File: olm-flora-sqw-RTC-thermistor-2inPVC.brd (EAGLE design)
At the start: 37.3 x 50.8 mm, 33 parts, among them IC1 ATMEGA32U4-AU, IC2 DS3231SN, IC3 MCP73831, IC4 MCP1700-33, J1 AYZ0202, X1 USBSMD, X3 8MHz

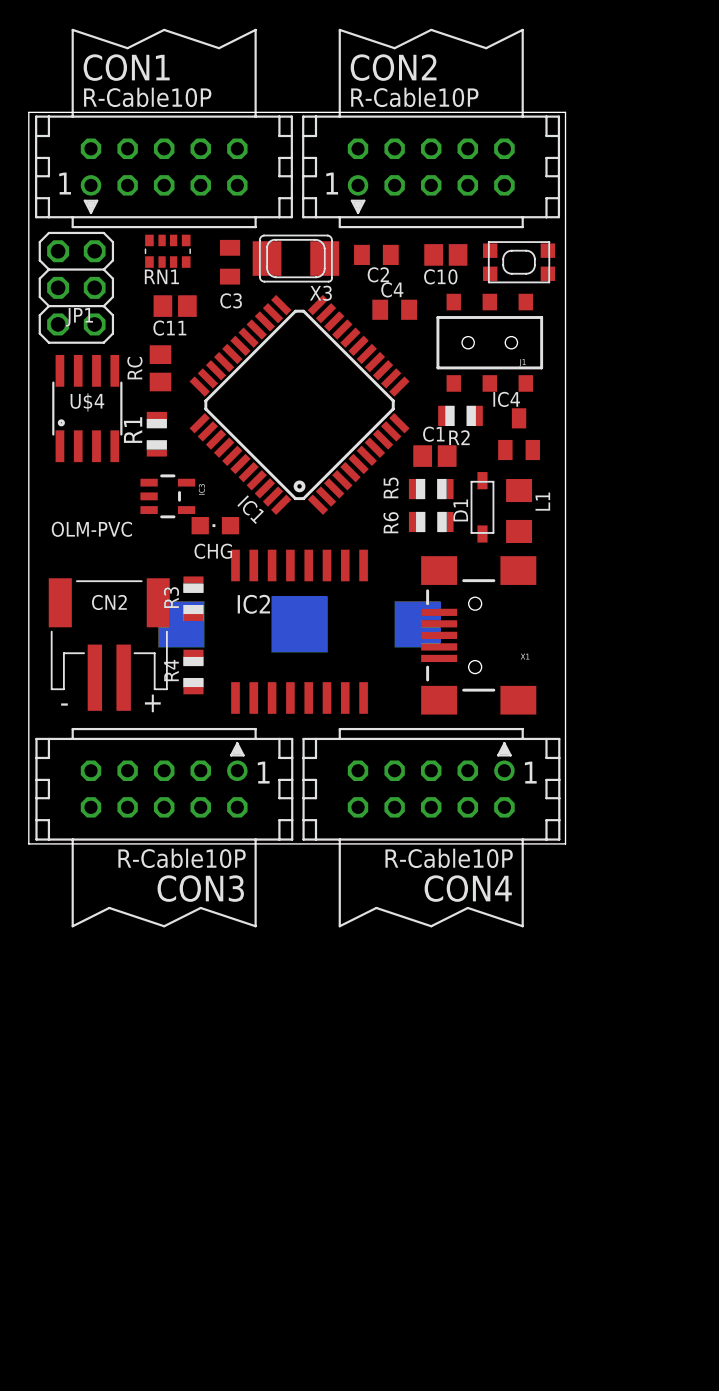
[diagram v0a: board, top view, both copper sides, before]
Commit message: update
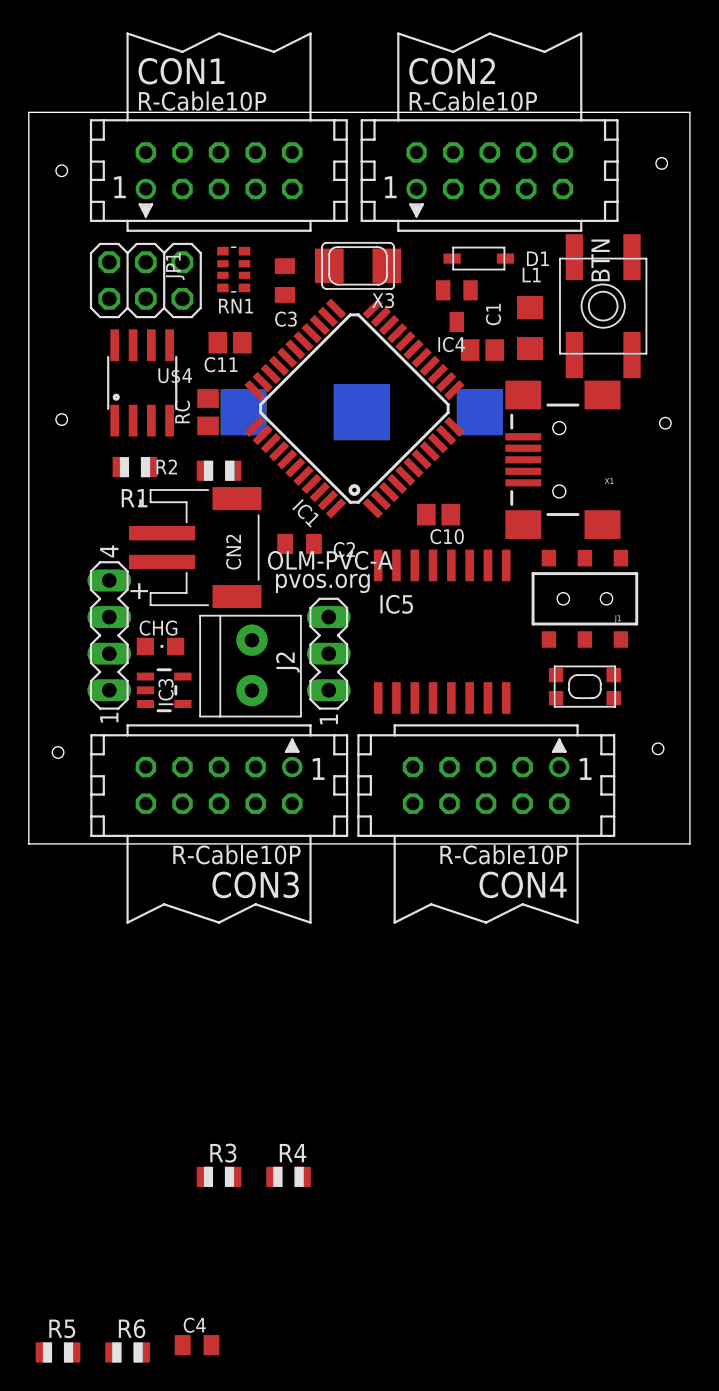
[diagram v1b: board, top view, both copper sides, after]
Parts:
- removed IC2: DS3231SN, comfile:SO16W
- added BTN: (no value), adafruit:EVQ-Q2
- added IC5: DS3231SN, comfile:SO16W
- added J2: 1X2-3.5MM, adafruit:1X2-3.5MM
- added SV1: (no value), con-lstb:MA03-1
- added SV2: (no value), con-lstb:MA04-1
- moved C4 73.2 mm to (11.7, -34.8)
- moved R5 65.3 mm to (2.03, -35.3)
- moved R6 61.4 mm to (6.86, -35.3), turned to 0 degrees
- moved R3 40.2 mm to (13.2, -23.1), turned to 0 degrees
- moved R4 35.7 mm to (18.0, -23.1), turned to 0 degrees
- moved BOOT 29.8 mm to (38.6, 10.9)
- moved C2 20.8 mm to (18.8, 20.8), turned to 0 degrees
- moved J1 19.0 mm to (38.6, 17.0)
- moved C10 18.0 mm to (28.4, 22.9), turned to 0 degrees
- moved D1 17.3 mm to (31.2, 40.6), turned to 0 degrees
- moved R2 17.2 mm to (13.2, 25.9)
- moved U$7 15.4 mm to (23.1, 30.0)
- moved X1 13.5 mm to (36.8, 26.7)
- moved IC3 13.5 mm to (9.40, 10.7)
- moved L1 12.7 mm to (34.8, 35.8)
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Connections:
- new net A0: IC1.36
- new net A1: IC1.37
- new net A2: IC1.38
- new net A3: IC1.39
- new net A4: IC1.40
- new net D11: IC1.12
- new net D4: BTN.B, BTN.B', IC1.25
- net 32KHZ: now also IC5.1; no longer IC2.1
- net D8: now also IC1.28
- net GND: now also BTN.A, BTN.A', IC5.10, IC5.11, IC5.12, IC5.13, IC5.5, IC5.6, IC5.7, IC5.8, IC5.9; no longer IC2.10, IC2.11, IC2.12, IC2.13, IC2.5, IC2.6, IC2.7, IC2.8, IC2.9
- net INT/SQW: now also IC5.3; no longer IC2.3
- net RST: now also IC5.4; no longer IC2.4
- net SCL: now also IC5.16; no longer IC2.16
- net SDA: now also IC5.15; no longer IC2.15
- net VBAT: now also IC5.14; no longer IC2.14
- net VCC: now also IC5.2; no longer IC2.2
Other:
- board size 37.3 x 50.8 mm -> 45.9 x 50.8 mm
- board text added: "OLM-PVC-A"
- board text added: "pvos.org"
- board text removed: "OLM-PVC"
